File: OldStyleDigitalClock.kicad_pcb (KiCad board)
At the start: 2 copper layers, 155 x 85 mm, 89 parts, among them J1 USB_A_OUT, J2 USB_A_OUT, J3 USB_C_IN, SW1 Set minutes, SW2 Set hours, U1 4071, U10 CD4026BE, U11 NE555D, U12 CD4060BE, U13 CD4017BE, U14 CD4017BE, U15 CD4017BE, U2 D168K, U3 CD4026BE, U4 D168K, U5 CD4026BE, U6 4073, U7 D168K, U8 CD4026BE, U9 D168K, Y1 HC49 XTAL (32768 Hz)

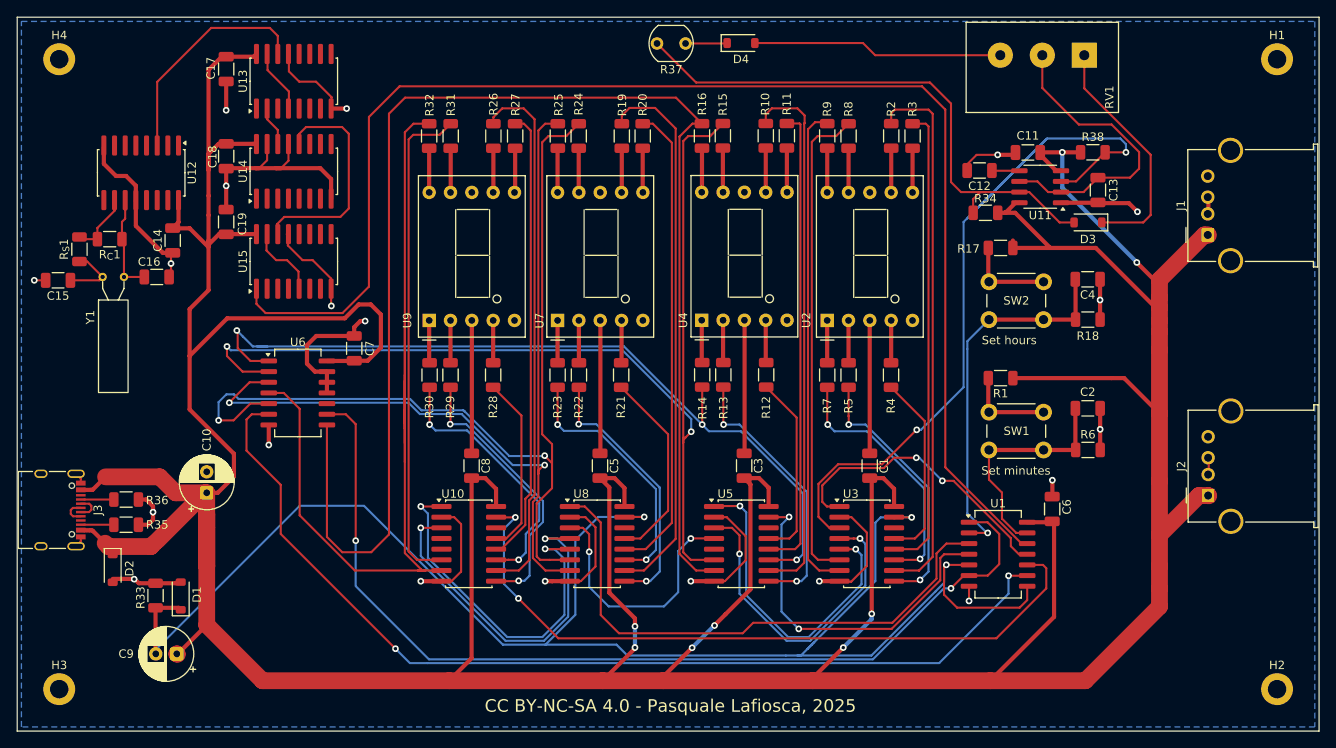
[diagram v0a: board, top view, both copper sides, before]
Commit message: Centering
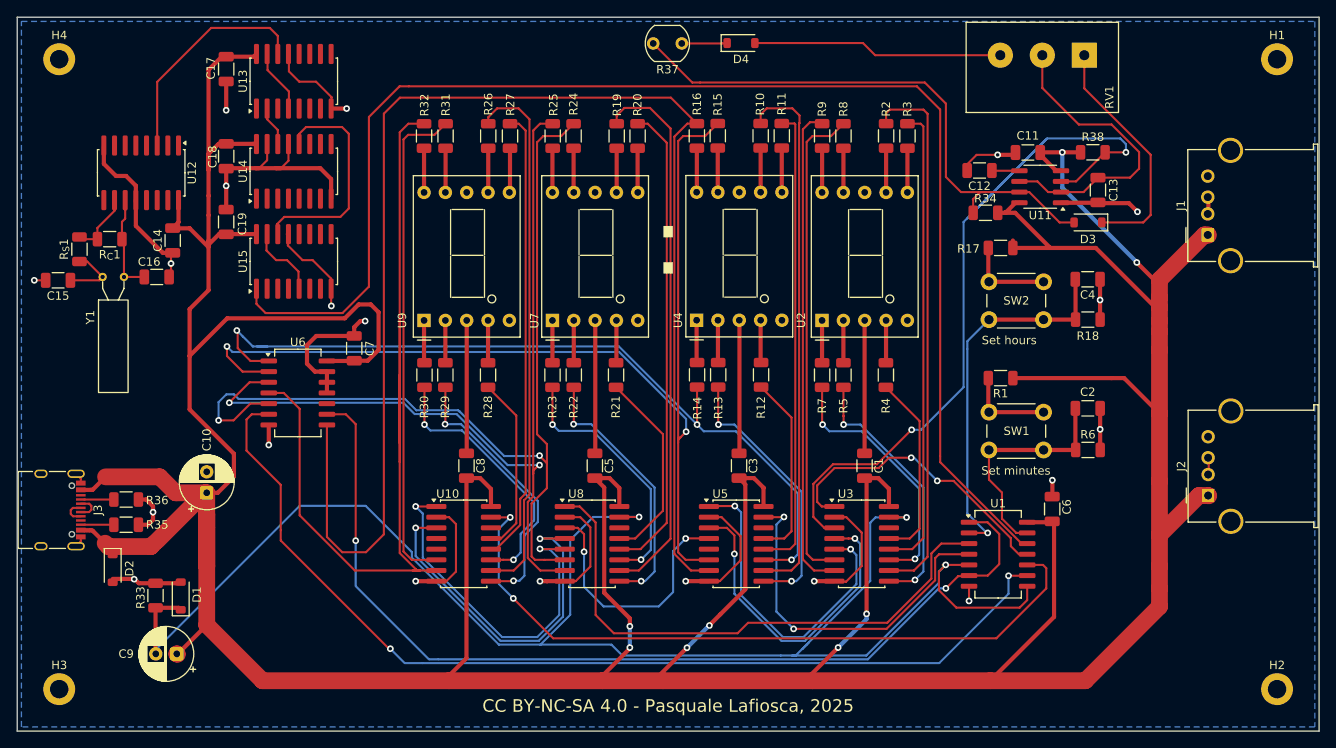
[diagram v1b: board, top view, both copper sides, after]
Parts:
- moved C1 0.61 mm to (150.9, 103.4)
- moved C3 0.61 mm to (135.9, 103.4)
- moved R15 0.61 mm to (133.4, 64.1)
- moved R16 0.61 mm to (130.9, 64.1)
- moved R19 0.61 mm to (121.4, 64.1)
- moved R2 0.61 mm to (153.5, 64.1)
- moved R21 0.61 mm to (121.3, 92.6)
- moved R3 0.61 mm to (156.0, 64.1)
- moved R7 0.61 mm to (145.8, 92.6)
- moved R9 0.61 mm to (145.8, 64.1)
- moved U3 0.61 mm to (150.5, 112.7)
- moved C5 0.61 mm to (118.8, 103.4)
- moved C8 0.61 mm to (103.5, 103.4)
- moved R20 0.61 mm to (123.9, 64.1)
- moved R22 0.61 mm to (116.3, 92.6)
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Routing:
- net MR: track 195.2 -> 196.1 mm
- net Net-(U5-G): track 169.7 -> 169.1 mm
- net Net-(U5-E): track 99.2 -> 98.6 mm
- net LED_PWM: track 96.4 -> 97.0 mm
- net Net-(U5-RESET): track 42.5 -> 43.2 mm
- net Net-(U10-RESET): track 85.4 -> 86.0 mm
- net Net-(U8-G): track 106.4 -> 105.8 mm
- net Net-(U8-F): track 112.4 -> 111.8 mm
- net Net-(U8-CLK): track 66.6 -> 67.2 mm
- net Net-(U5-F): track 127.9 -> 127.3 mm
- net Net-(U3-CLK): track 35.3 -> 35.9 mm
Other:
- board text added: ":"
